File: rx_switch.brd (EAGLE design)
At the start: 100 x 80 mm, 9 parts, among them IC1 AT90S2313S

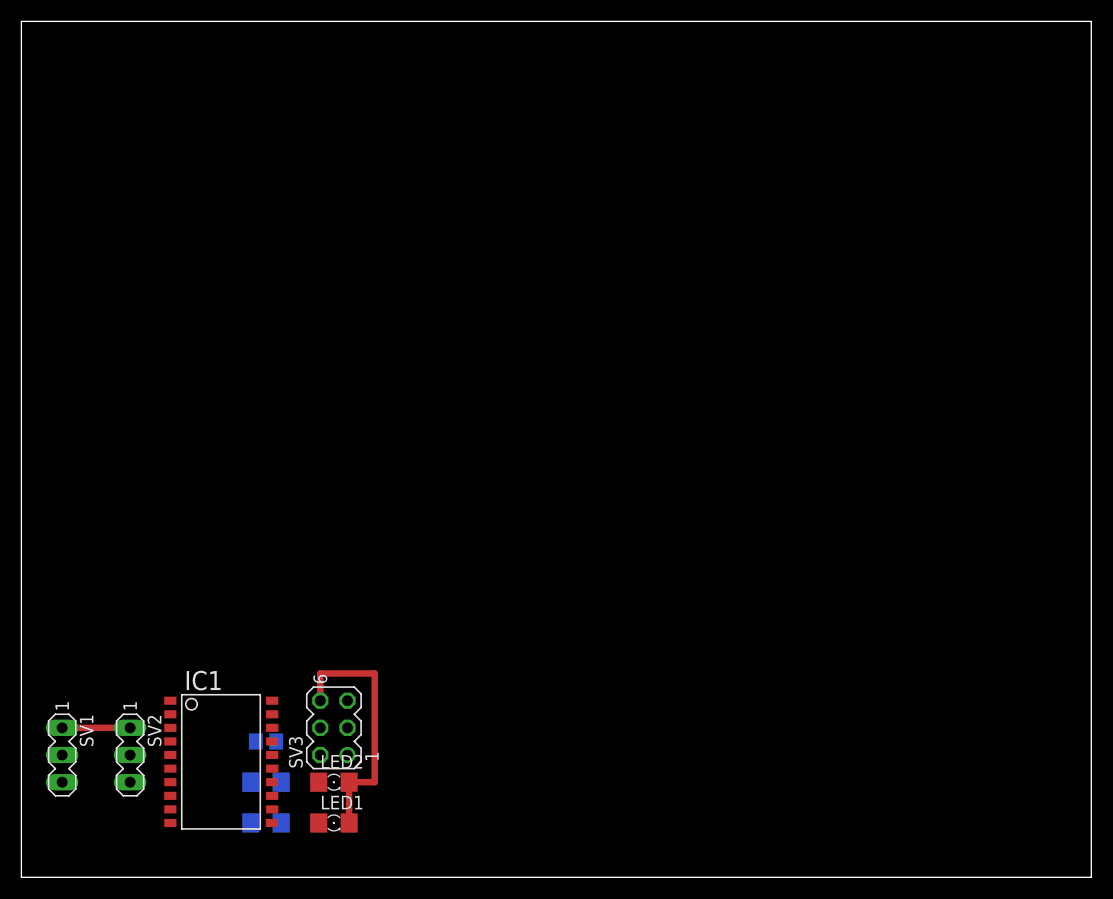
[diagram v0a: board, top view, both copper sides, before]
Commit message: PCB design
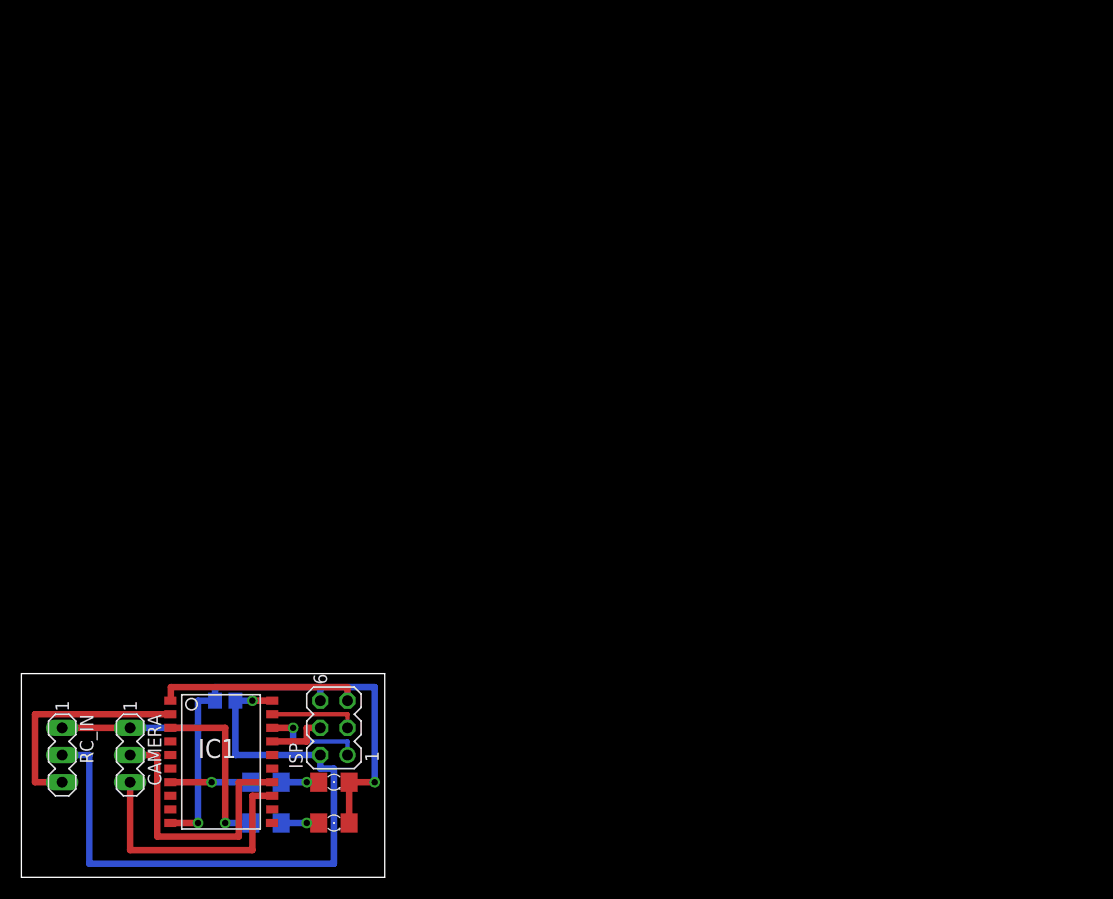
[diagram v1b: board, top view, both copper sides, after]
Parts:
- CAMERA: value CAMERA -> (none)
- IC1: value AT90S2313S -> (none)
- ISP: value ISP -> (none)
- RC_IN: value RC IN -> (none)
- moved C2 5.39 mm to (19.1, 16.5)
- renumbered SV1 to RC_IN, SV2 to CAMERA, SV3 to ISP
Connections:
- net N$7 renamed ISP
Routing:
- net VCC: track 0.00 -> 63.5 mm, vias 0 -> 1
- net GND: track 30.3 -> 60.9 mm, vias 0 -> 2
- net N$4: track 0.00 -> 26.0 mm
- net N$5: track 0.00 -> 24.7 mm
- net N$3: track 0.00 -> 21.5 mm
- net N$1: track 0.00 -> 19.1 mm
- net N$10: track 0.00 -> 16.4 mm, vias 0 -> 1
- net N$6: track 0.00 -> 9.58 mm, vias 0 -> 1
- net ISP: track 0.00 -> 8.31 mm
- net N$9: track 0.00 -> 7.52 mm, vias 0 -> 1
- net N$2: track 0.00 -> 5.77 mm
- net N$8: track 0.00 -> 3.51 mm, vias 0 -> 1
- net N$11: track 0.00 -> 3.51 mm, vias 0 -> 1
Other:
- board size 100 x 80 mm -> 34 x 19 mm
- board text added: "Janne Mäntyharju (c) 2013"
- board text added: "NXShutter"
- board text added: "V 2.0"
